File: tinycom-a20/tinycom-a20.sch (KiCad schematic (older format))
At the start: 38 parts, among them P1 CONN_02X08, P2 CONN_02X08, U1 ALLWINNERA10/TFBGA441, U2 H5TQG63BFR/FBGA96, U3 H27UBG8T2A/TSOP48, U4 H5TQG63BFR/FBGA96, Y1 Crystal_Small, Y2 Crystal_Small

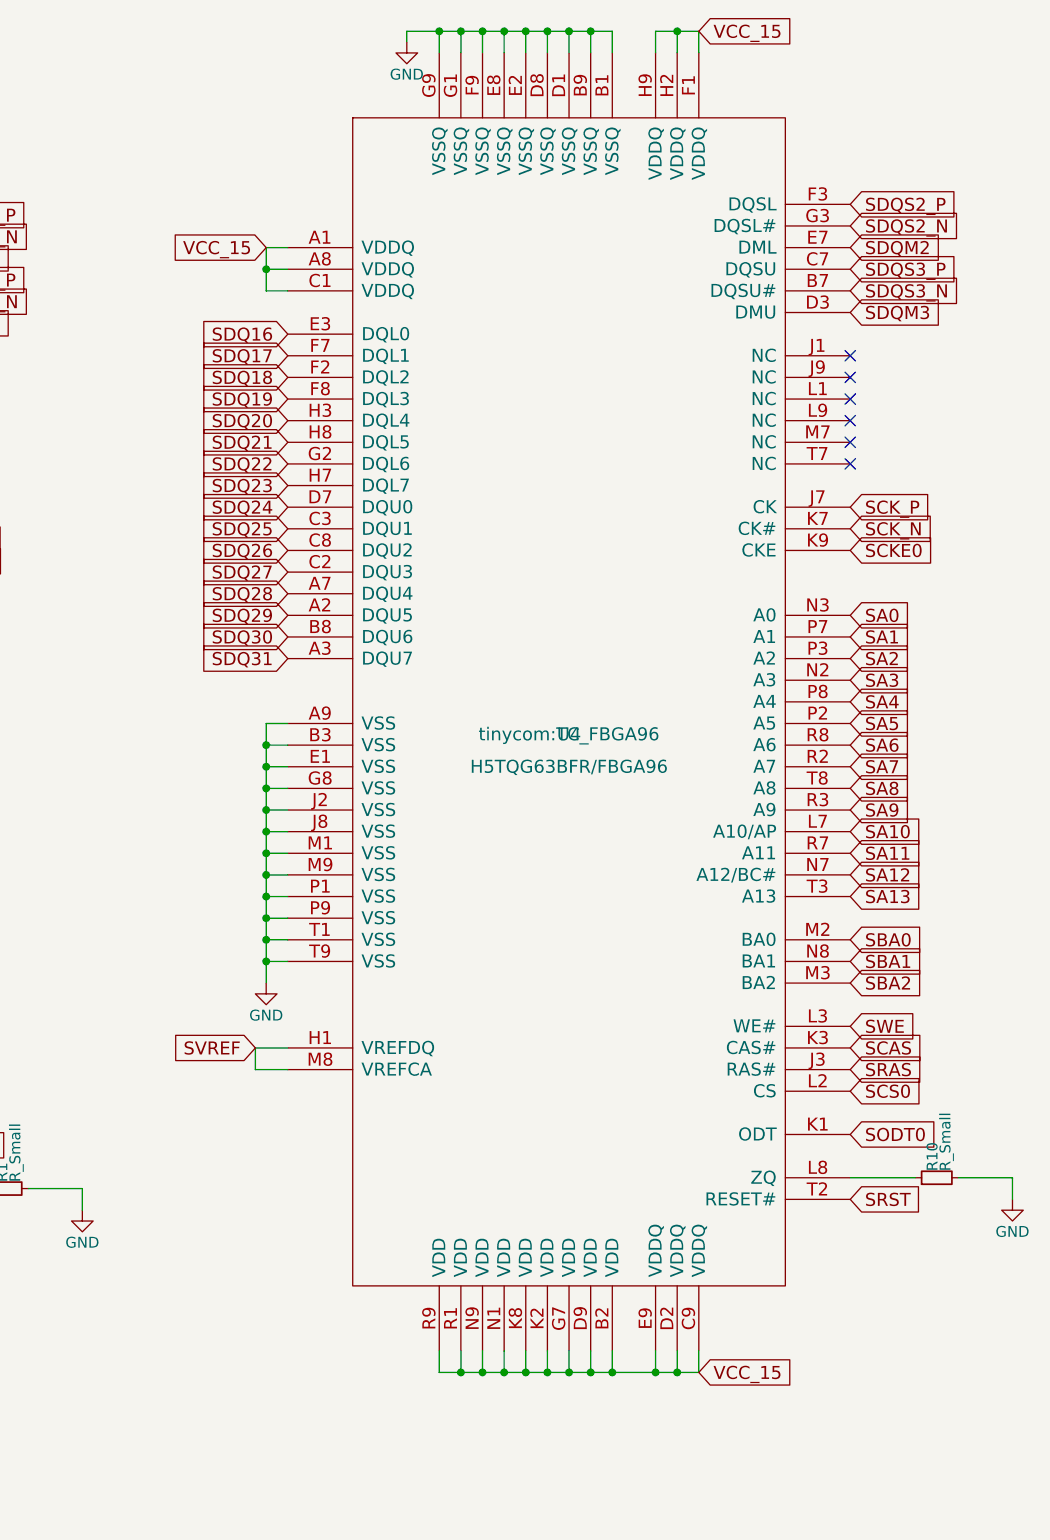
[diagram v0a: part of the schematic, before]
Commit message: before import routes
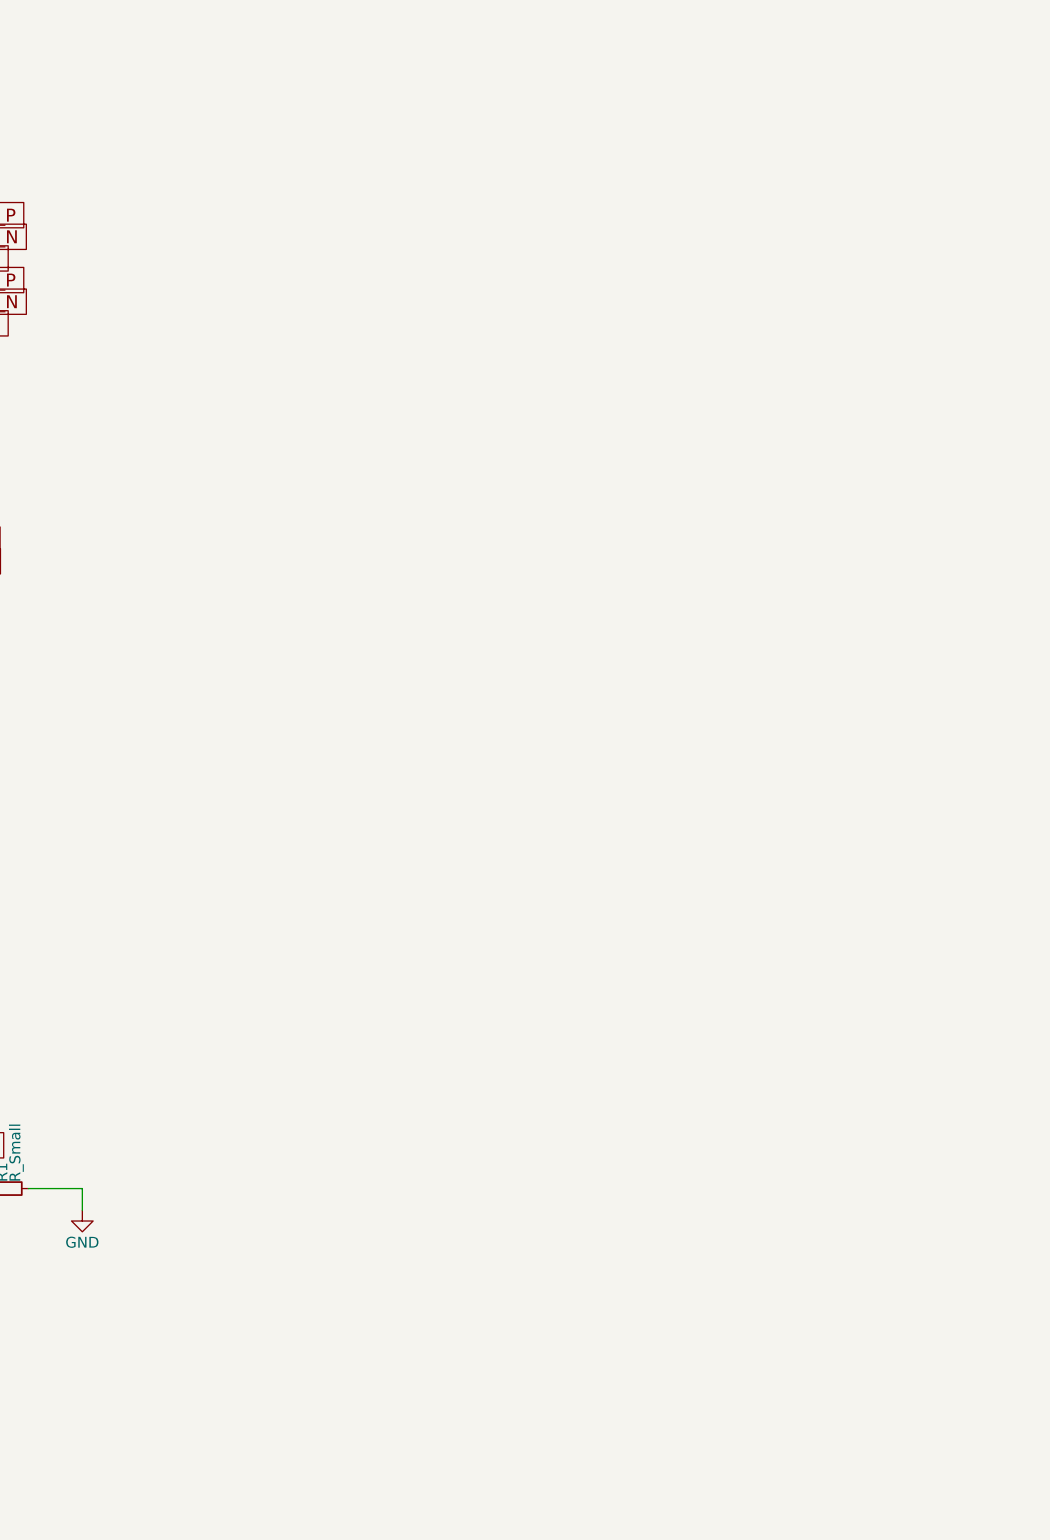
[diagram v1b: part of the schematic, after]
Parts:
- removed R10: R_Small, Resistors_SMD:R_0603, symbol R_Small
- removed U4: H5TQG63BFR/FBGA96, tinycom:TC_FBGA96, symbol H5TQG63BFR/FBGA96
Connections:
- no-connect marks 239 -> 233
